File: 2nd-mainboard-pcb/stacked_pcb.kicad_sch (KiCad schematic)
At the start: 20 parts, among them J16 Steckverbinder_Male_Fans, J17 Steckverbinder_Male_Leistung, J18 Steckverbinder_Female_Leistung, J19 Steckverbinder_Male_Motoren, J20 Steckverbinder_Female_Motoren, J24 Steckverbinder_Male_Fans, J25 HLE-107-02-L-DV, J26 Steckverbinder_Male_Leistung

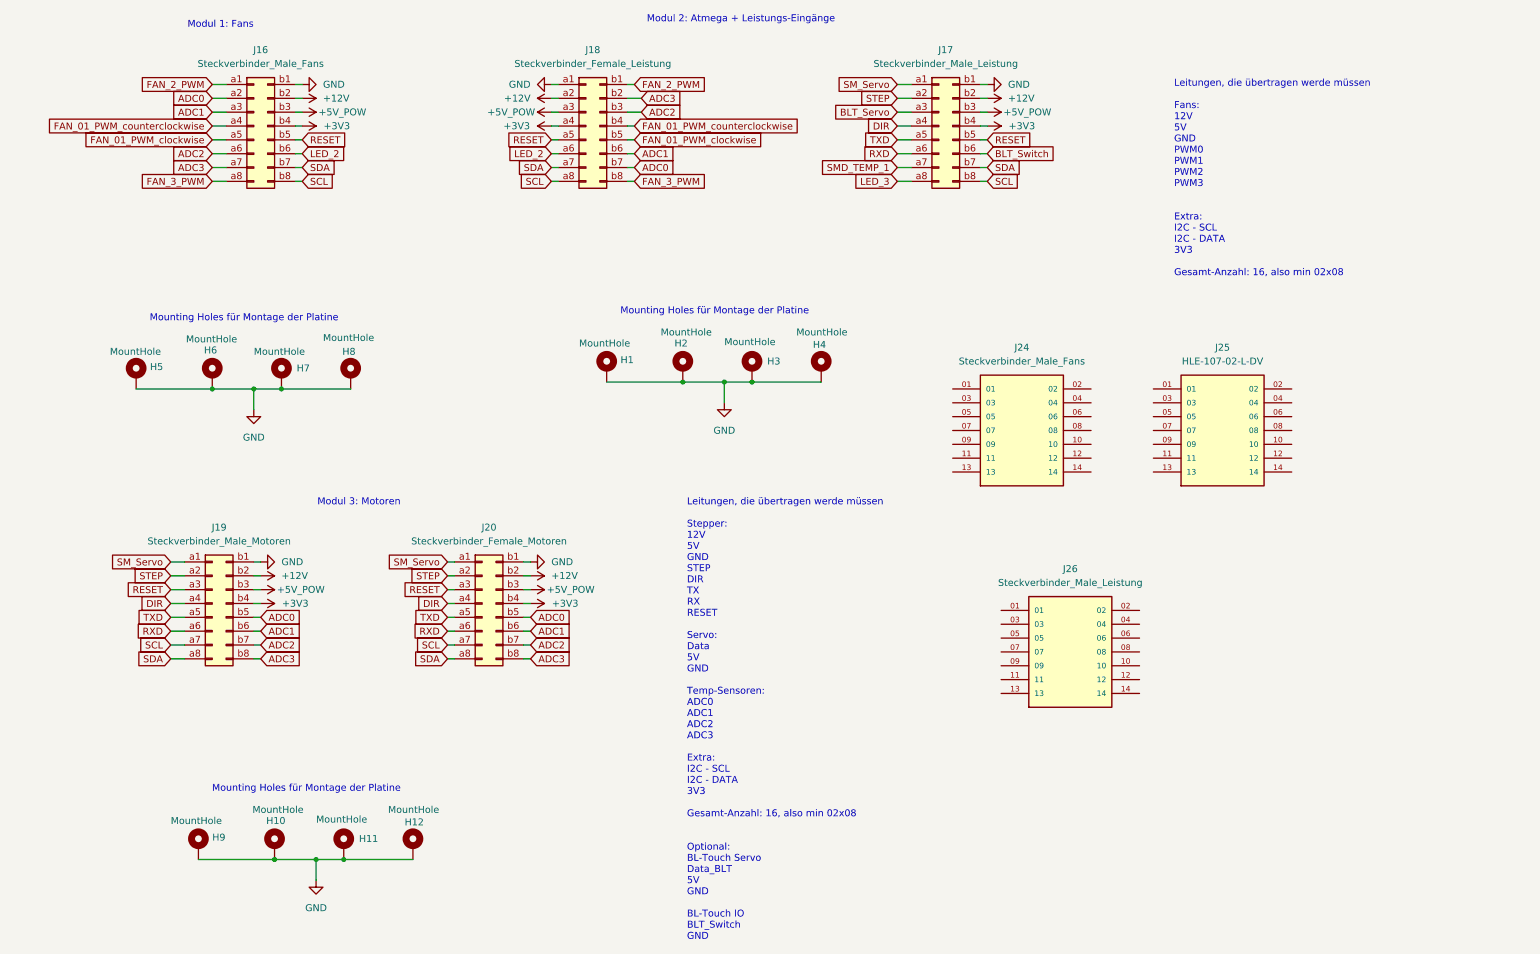
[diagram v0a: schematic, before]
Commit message: Fan-PCB-Beginning
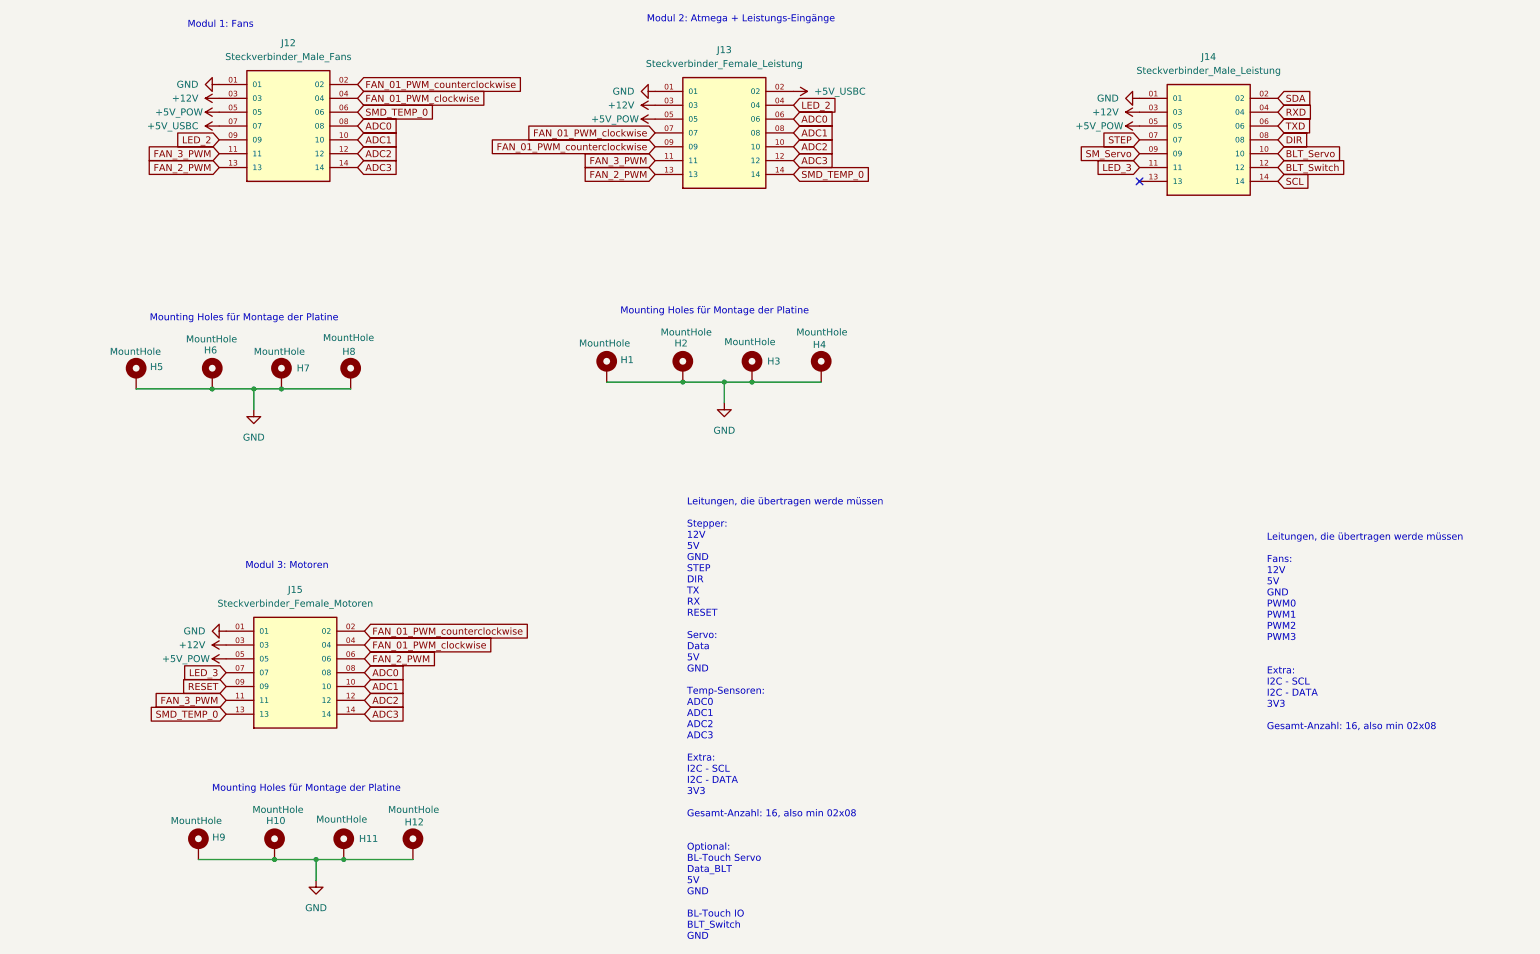
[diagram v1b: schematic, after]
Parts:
- removed J16: Steckverbinder_Male_Fans, CustomFotLibByJan:BF100-16-A-D-1-0640-L-C, symbol Connector_Generic:Conn_02x08_Row_Letter_First
- removed J17: Steckverbinder_Male_Leistung, CustomFotLibByJan:BF100-16-A-D-1-0640-L-C, symbol Connector_Generic:Conn_02x08_Row_Letter_First
- removed J18: Steckverbinder_Female_Leistung, CustomFotLibByJan:BF030-16A-B1-0360-0277-0600-LB, symbol Connector_Generic:Conn_02x08_Row_Letter_First
- removed J19: Steckverbinder_Male_Motoren, CustomFotLibByJan:BF100-16-A-D-1-0640-L-C, symbol Connector_Generic:Conn_02x08_Row_Letter_First
- removed J20: Steckverbinder_Female_Motoren, CustomFotLibByJan:BF030-16A-B1-0360-0277-0600-LB, symbol Connector_Generic:Conn_02x08_Row_Letter_First
- added J15: Steckverbinder_Female_Motoren, Imported_Component_Footprints:SAMTEC_HLE-107-02-L-DV, symbol Imported_Component_Symbols:HLE-107-02-L-DV
- J13: renamed from J25; value HLE-107-02-L-DV -> Steckverbinder_Female_Leistung
- renumbered J24 to J12, J26 to J14
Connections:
- net +12V: now also J12.03, J13.03, J14.03, J15.03
- net +5V_POW: now also J12.05, J13.05, J14.05, J15.05
- net ADC0: now also J12.08, J13.06, J15.08
- net ADC1: now also J12.10, J13.08, J15.10
- net ADC2: now also J12.12, J13.10, J15.12
- net ADC3: now also J12.14, J13.12, J15.14
- net BLT_Servo: now also J14.10
- net BLT_Switch: now also J14.12
- net DIR: now also J14.08
- net FAN_01_PWM_clockwise: now also J12.04, J13.07, J15.04
- net FAN_01_PWM_counterclockwise: now also J12.02, J13.09, J15.02
- net FAN_2_PWM: now also J12.13, J13.13, J15.06
- net FAN_3_PWM: now also J12.11, J13.11, J15.11
- net GND: now also J12.01, J13.01, J14.01, J15.01
- net LED_2: now also J12.09, J13.04
- net LED_3: now also J14.11, J15.07
- net RESET: now also J15.09
- net RXD: now also J14.04
- net SCL: now also J14.14
- net SDA: now also J14.02
- net SM_Servo: now also J14.09
- net STEP: now also J14.07
- net TXD: now also J14.06
- net SMD_TEMP_0: now reaches J12.06
- net SMD_TEMP_0: now also J13.14, J15.13
- net +5V_USBC: now reaches J12.07
- net +5V_USBC: now also J13.02
- no-connect marks 0 -> 1
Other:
- moved on the sheet: J12, J13, J14
